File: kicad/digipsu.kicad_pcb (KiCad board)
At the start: 2 copper layers, 137.2 x 174 mm, 154 parts, among them J1 Screw_Terminal_01x03, J2 PWR IN, J3 8P8C, J4 8P8C, J5 8P8C, Q1 BC327, Q2 BC337, Q3 2N6058, Q4 2N6058, Q5 IRLZ34N, SW1 RotaryEncoder_Switch, SW2 RotaryEncoder_Switch, U1 INA169, U10 Pico, U11 M24C32-RMN, U12 SN75176BP, U13 6N137, U14 SN75176BP, U15 SN75176BP, U16 74AC14, U2 MCP6002-xP, U3 Pico, U301 74AC14, U4 MCP6002-xP, U5 L7805, U6 MCP3464R, U7 LF33_TO220, U8 6N137, U9 SN75176BP

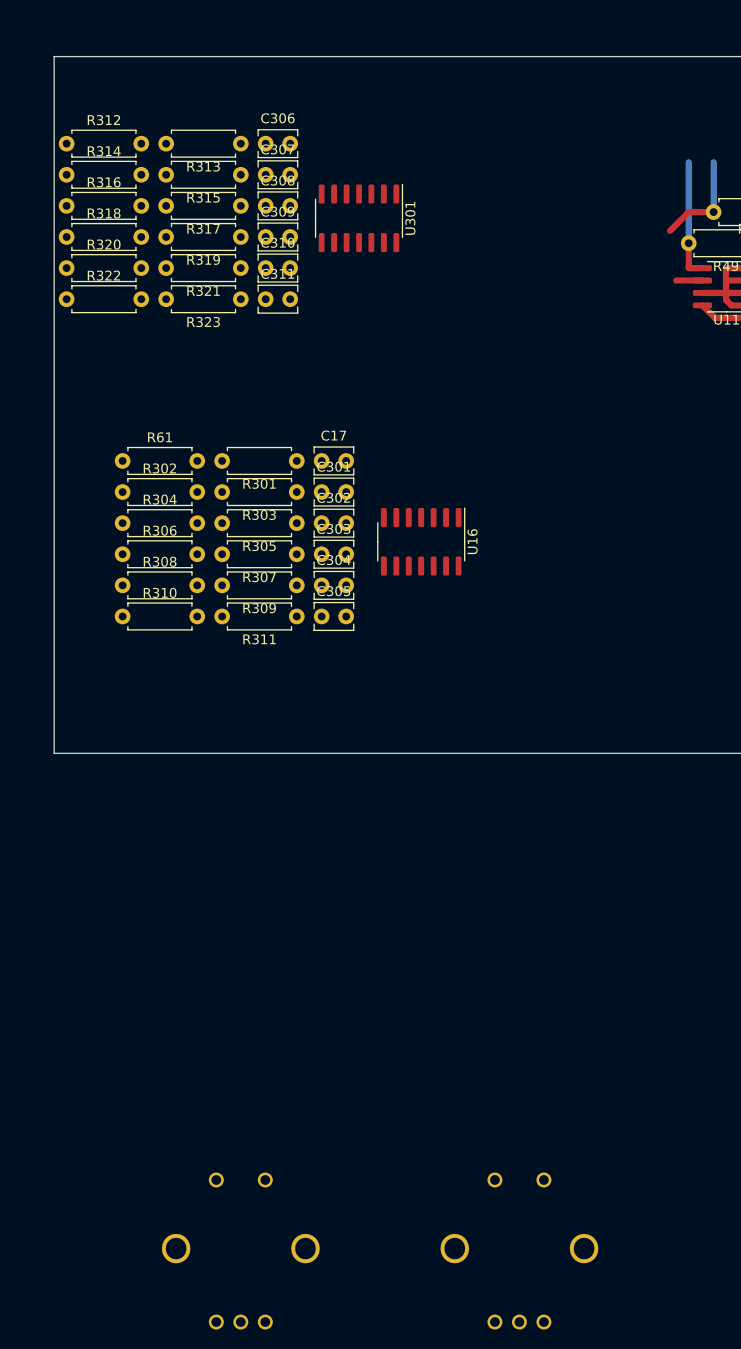
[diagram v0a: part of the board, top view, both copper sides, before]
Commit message: Compile gerber and drill files in one zip
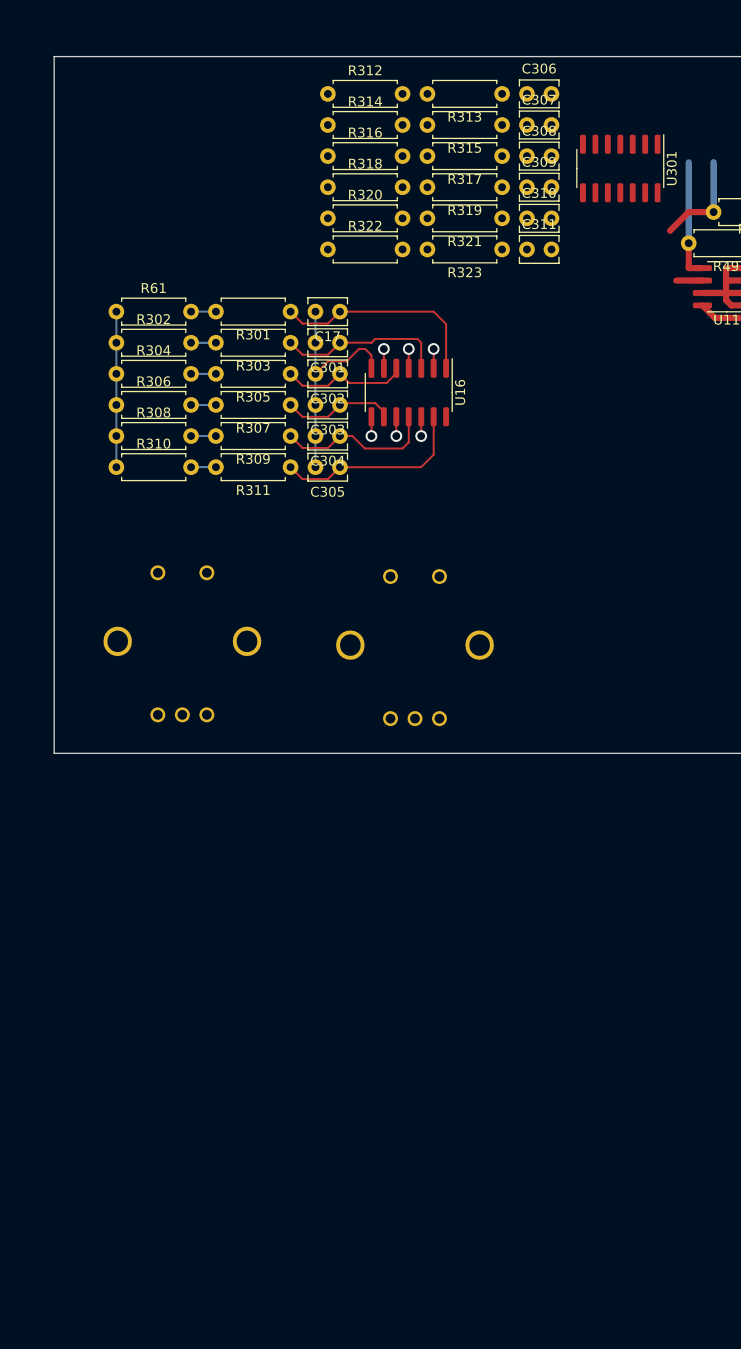
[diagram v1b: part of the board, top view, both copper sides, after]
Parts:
- moved SW1 62.5 mm to (57.1, 192.0)
- moved SW2 62.3 mm to (33.4, 191.7)
- moved C307 27.1 mm to (66.0, 131.4)
- moved C309 27.1 mm to (66.0, 137.8)
- moved C310 27.1 mm to (66.0, 141.0)
- moved C306 27.1 mm to (66.0, 128.3)
- moved C308 27.1 mm to (66.0, 134.6)
- moved C311 27.1 mm to (66.0, 144.1)
- moved R315 27.1 mm to (63.5, 131.4)
- moved R319 27.1 mm to (63.5, 137.8)
- moved R321 27.1 mm to (63.5, 141.0)
- moved R314 27.1 mm to (45.7, 131.4)
- moved R318 27.1 mm to (45.7, 137.8)
- moved R320 27.1 mm to (45.7, 141.0)
- moved R313 27.1 mm to (63.5, 128.3)
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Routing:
- net /User Interface/GND: track 0.00 -> 24.2 mm
- net Net-(C17-Pad1): track 0.00 -> 21.9 mm
- net Net-(C305-Pad1): track 0.00 -> 20.0 mm
- net Net-(C301-Pad1): track 0.00 -> 17.3 mm
- net Net-(C304-Pad1): track 0.00 -> 16.5 mm
- net +3.3V: track 25.0 -> 40.9 mm
- net Net-(C302-Pad1): track 0.00 -> 13.1 mm
- net Net-(C303-Pad1): track 0.00 -> 11.5 mm
- net /User Interface/SWin6: track 0.00 -> 2.54 mm
- net /User Interface/SWin5: track 0.00 -> 2.54 mm
- net /User Interface/SWin4: track 0.00 -> 2.54 mm
- net /User Interface/SWin3: track 0.00 -> 2.54 mm
- net /User Interface/SWin2: track 0.00 -> 2.54 mm
- net /User Interface/SWin1: track 0.00 -> 2.54 mm
- net /User Interface/SWout6: track 0.00 -> 1.97 mm, vias 0 -> 1
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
